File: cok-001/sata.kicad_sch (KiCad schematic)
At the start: 89 parts, among them J3401 Conn_01x22_Pin, Q3401 DTC144E, Q3402 DTC144E, Q3403 DTC144E, Q3404 DTC144E, Y3402 25MHz

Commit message: update 10
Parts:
- U3401: value ~ -> (none)

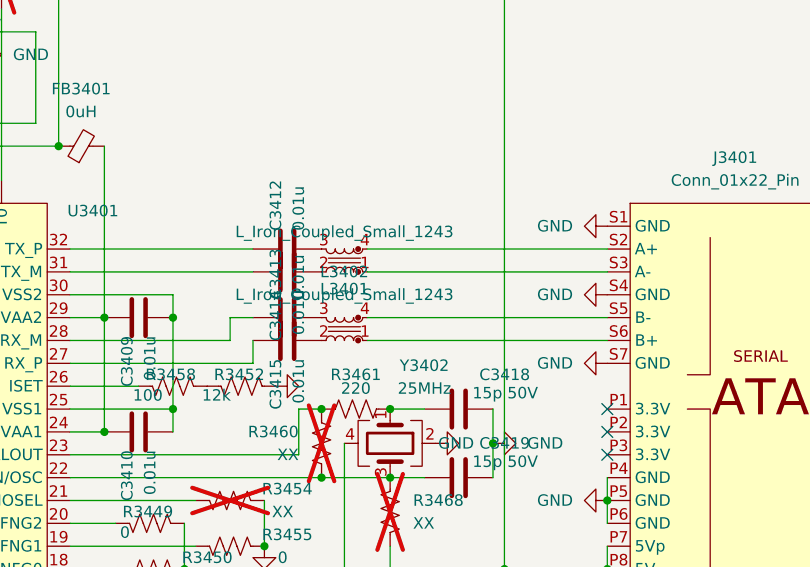
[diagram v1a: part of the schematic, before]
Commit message: lf
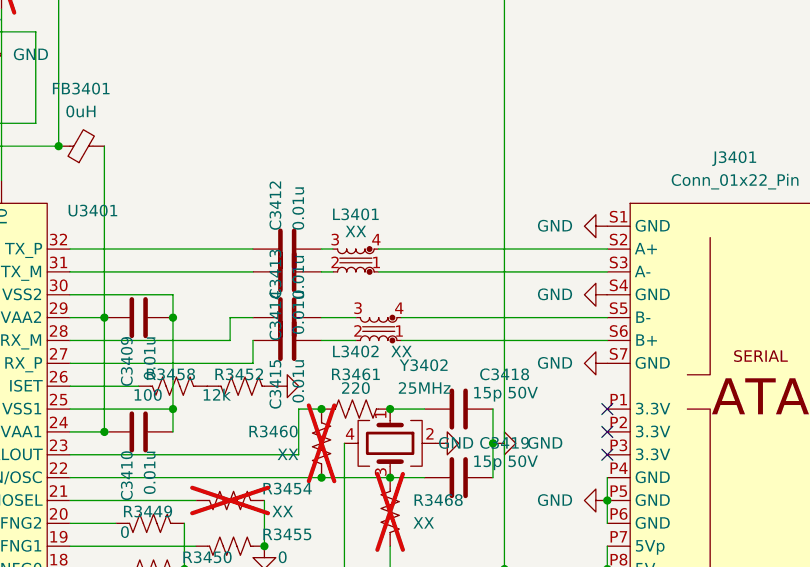
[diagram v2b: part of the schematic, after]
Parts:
- L3401, L3402: value L_Iron_Coupled_Small_1243 -> XX
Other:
- moved on the sheet: L3401, L3402
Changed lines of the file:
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@@
 	(wire
 		(pts
-			(xy 157.48 90.17) (xy 184.15 90.17)
+			(xy 158.75 90.17) (xy 184.15 90.17)
 		)
 		(stroke
@@
 	(wire
 		(pts
-			(xy 157.48 97.79) (xy 184.15 97.79)
+			(xy 161.29 97.79) (xy 184.15 97.79)
 		)
 		(stroke
@@
 	(wire
 		(pts
+			(xy 153.67 87.63) (xy 152.4 87.63)
+		)
+		(stroke
+			(width 0)
+			(type default)
+		)
+	)
+	(wire
+		(pts
 			(xy 114.3 172.72) (xy 114.3 139.7)
 		)
@@
 	(wire
 		(pts
-			(xy 157.48 95.25) (xy 184.15 95.25)
+			(xy 153.67 90.17) (xy 152.4 90.17)
+		)
+		(stroke
+			(width 0)
+			(type default)
+		)
+	)
+	(wire
+		(pts
+			(xy 161.29 95.25) (xy 184.15 95.25)
 		)
 		(stroke
@@
 	(wire
 		(pts
+			(xy 156.21 97.79) (xy 152.4 97.79)
+		)
+		(stroke
+			(width 0)
+			(type default)
+		)
+	)
+	(wire
+		(pts
 			(xy 66.04 53.34) (xy 73.66 53.34)
 		)
@@
 	(wire
 		(pts
-			(xy 157.48 87.63) (xy 184.15 87.63)
+			(xy 158.75 87.63) (xy 184.15 87.63)
 		)
 		(stroke
@@
 	(wire
 		(pts
+			(xy 156.21 95.25) (xy 152.4 95.25)
+		)
+		(stroke
+			(width 0)
+			(type default)
+		)
+	)
+	(wire
+		(pts
 			(xy 109.22 53.34) (xy 111.76 53.34)
 		)
@@
 	(symbol
 		(lib_id "Device:L_Iron_Coupled_Small_1243")
-		(at 154.94 88.9 180)
+		(at 156.21 88.9 180)
 		(unit 1)
 		(body_style 1)
@@
 		(dnp no)
 		(property "Reference" "L3401"
-			(at 154.94 92.075 0)
+			(at 156.21 83.82 0)
 			(show_name no)
 			(do_not_autoplace no)
@@
 			)
 		)
-		(property "Value" "L_Iron_Coupled_Small_1243"
-			(at 154.94 85.725 0)
+		(property "Value" "XX"
+			(at 156.21 85.725 0)
 			(show_name no)
 			(do_not_autoplace no)
@@
 		)
 		(property "Footprint" "Inductor_SMD:L_CommonModeChoke_Coilcraft_0805USB"
-			(at 154.94 88.9 0)
+			(at 156.21 88.9 0)
 			(hide yes)
 			(show_name no)
@@
 		)
 		(property "Datasheet" ""
-			(at 154.94 88.9 0)
+			(at 156.21 88.9 0)
 			(hide yes)
 			(show_name no)
@@
 		)
 		(property "Description" "Coupled inductor with iron core, small symbol"
-			(at 154.94 88.9 0)
+			(at 156.21 88.9 0)
 			(hide yes)
 			(show_name no)
@@
 	(symbol
 		(lib_id "Device:L_Iron_Coupled_Small_1243")
-		(at 154.94 96.52 180)
+		(at 158.75 96.52 180)
 		(unit 1)
 		(body_style 1)
@@
 		(in_pos_files yes)
 		(dnp no)
-		(fields_autoplaced yes)
 		(property "Reference" "L3402"
-			(at 154.94 90.17 0)
+			(at 156.21 99.06 0)
 			(show_name no)
 			(do_not_autoplace no)
@@
 			)
 		)
-		(property "Value" "L_Iron_Coupled_Small_1243"
-			(at 154.94 92.71 0)
+		(property "Value" "XX"
+			(at 161.29 99.06 0)
 			(show_name no)
 			(do_not_autoplace no)
@@
 		)
 		(property "Footprint" "Inductor_SMD:L_CommonModeChoke_Coilcraft_0805USB"
-			(at 154.94 96.52 0)
+			(at 158.75 96.52 0)
 			(hide yes)
 			(show_name no)
@@
 		)
 		(property "Datasheet" ""
-			(at 154.94 96.52 0)
+			(at 158.75 96.52 0)
 			(hide yes)
 			(show_name no)
@@
 		)
 		(property "Description" "Coupled inductor with iron core, small symbol"
-			(at 154.94 96.52 0)
+			(at 158.75 96.52 0)
 			(hide yes)
 			(show_name no)
